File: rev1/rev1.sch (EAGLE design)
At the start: 34 parts, among them IC1 ATMEGA168-AU, IC3 74AHC1G04DBV, Q1 MOSFET-NCHANNEL-IRLR3705ZPBF, Y1 16MHz

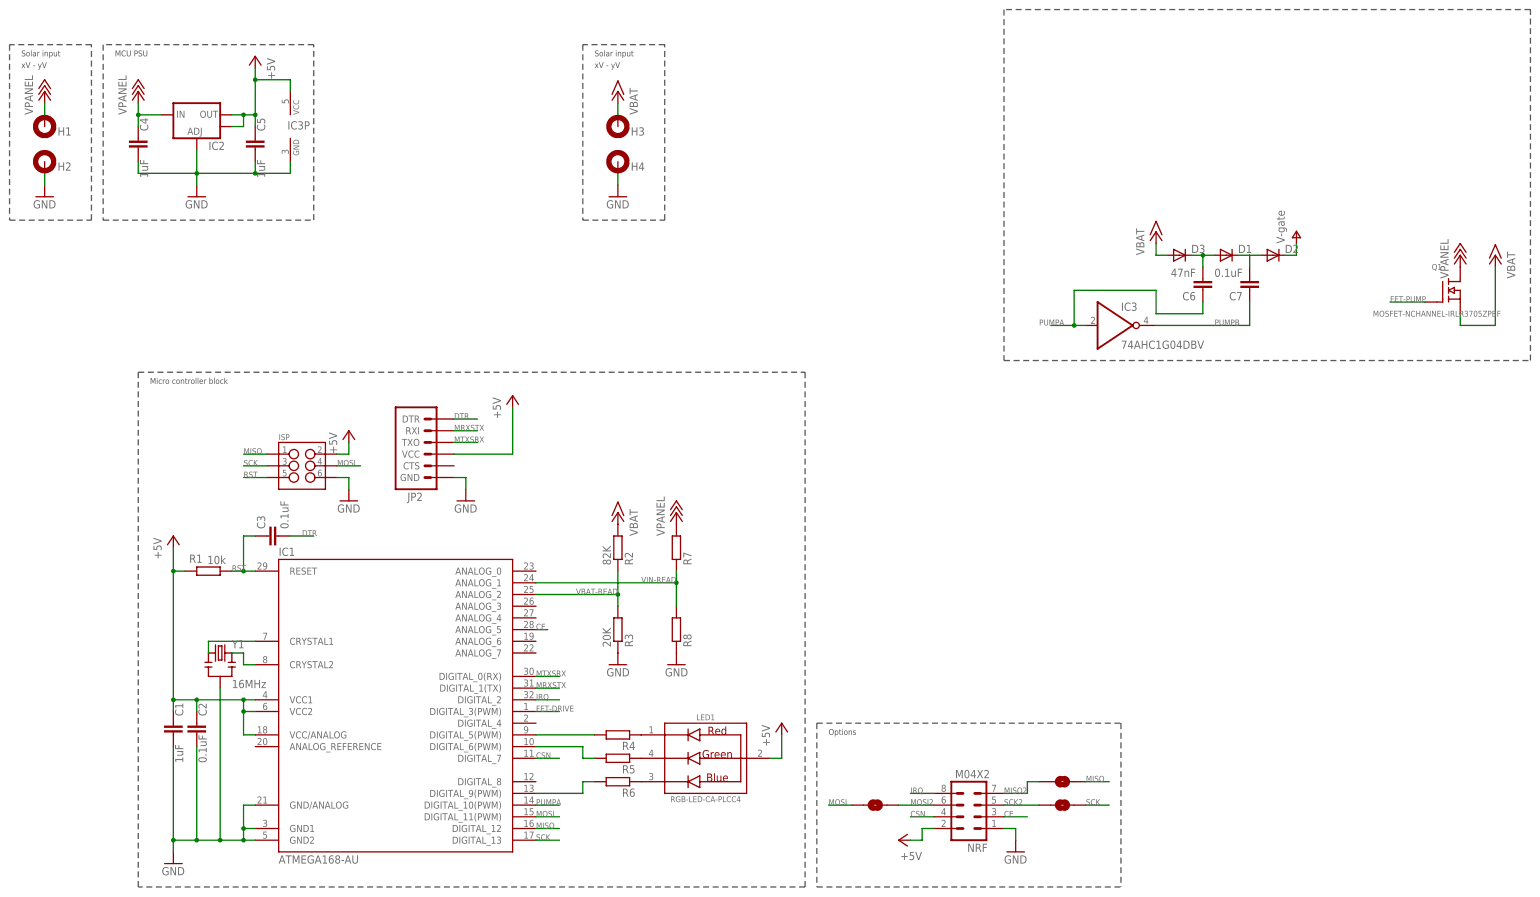
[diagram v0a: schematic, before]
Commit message: Schematic pre-finished. Needs values added
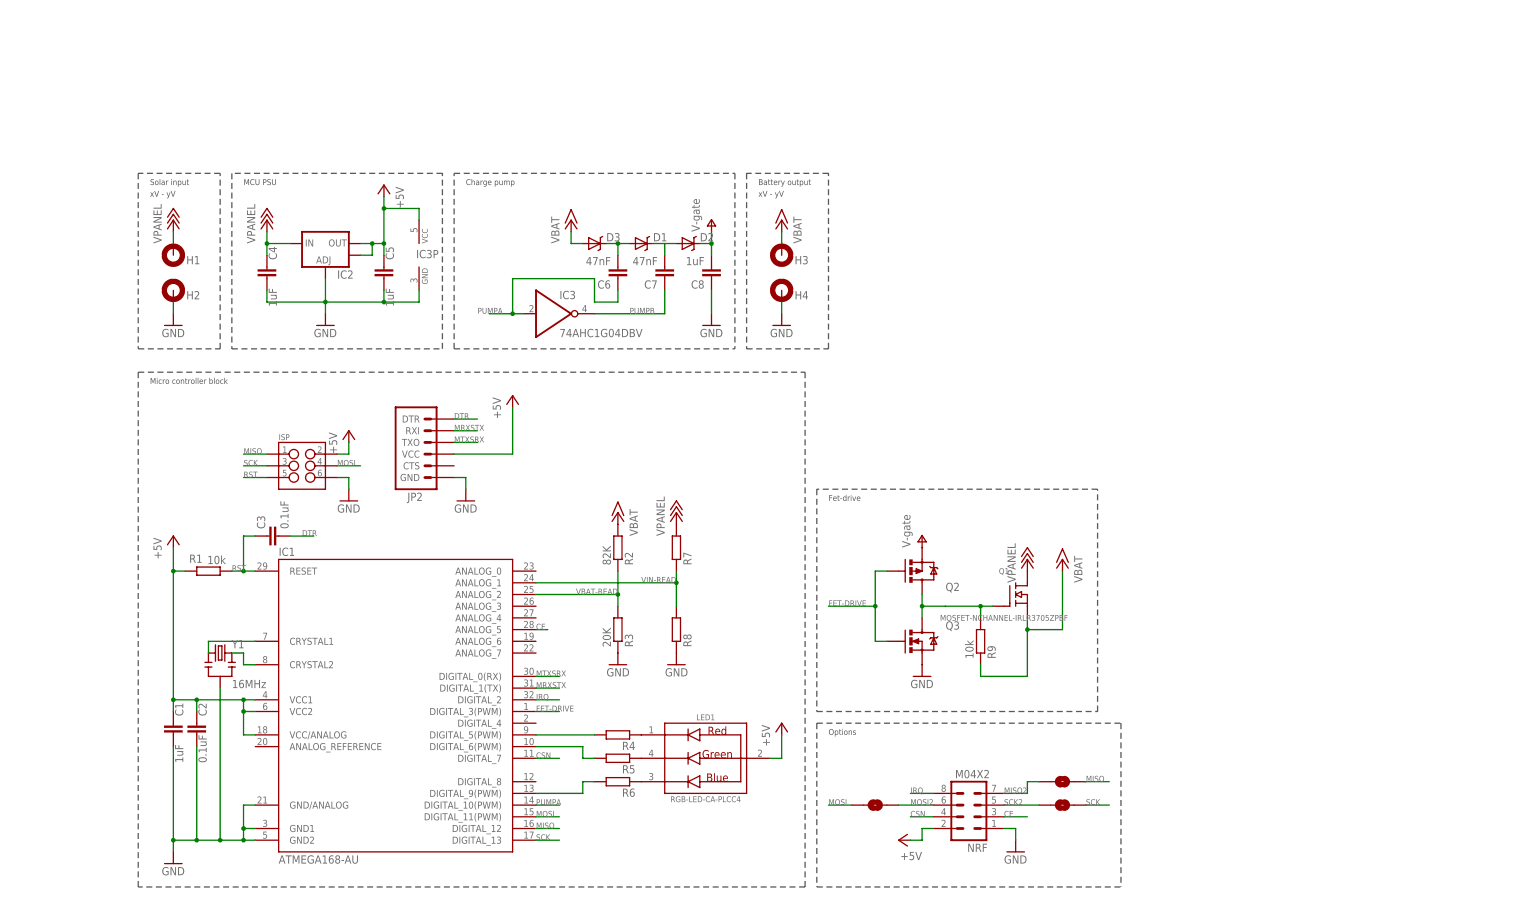
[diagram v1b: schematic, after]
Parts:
- added C8: 1uF, resistor:C-EUC0603K
- added Q2: MOSFET-PCHANNELSMD, SparkFun-DiscreteSemi:MOSFET-PCHANNELSMD
- added Q3: MOSFET-NCHANNELBSS138, SparkFun-DiscreteSemi:MOSFET-NCHANNELBSS138
- added R9: 10k, resistor:R-EU_R0603
- C7: value 0.1uF -> 47nF
- D1, D2, D3: value (none) -> DIODE-SCHOTTKY; device SparkFun-DiscreteSemi:DIODESOD -> SparkFun-DiscreteSemi:DIODE-SCHOTTKY
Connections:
- new net N$28: Q2.D, Q3.D
- net +15V: now also R9.1
- net FET-DRIVE: now also Q2.G, Q3.G
- net FET-PUMP: now also R9.2
- net GND: now also C8.1, Q3.S
- net V+: now also C8.2, Q2.S
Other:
- note added: "Battery output"
- note added: "Charge pump"
- note added: "Fet-drive"
- moved on the sheet: C4, C5, C6, C7, H1, H2, H3, H4, IC2, IC3, IC3P, Q1
